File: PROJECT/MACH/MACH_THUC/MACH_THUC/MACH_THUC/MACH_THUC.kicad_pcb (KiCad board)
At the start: 2 copper layers, 177.8 x 99.1 mm, 66 parts, among them K1 SANYOU_SRD_Form_C, K2 SANYOU_SRD_Form_C, Q1 2SB688, Q2 BC547, Q3 BC547, U1 LM7805_TO220, U2 DS1307+, U3 LCD-016N002L, U4 PCF8574, U5 PC817, U6 PC817, Y1 Crystal 20M, Y2 Crystal 32.768KHz

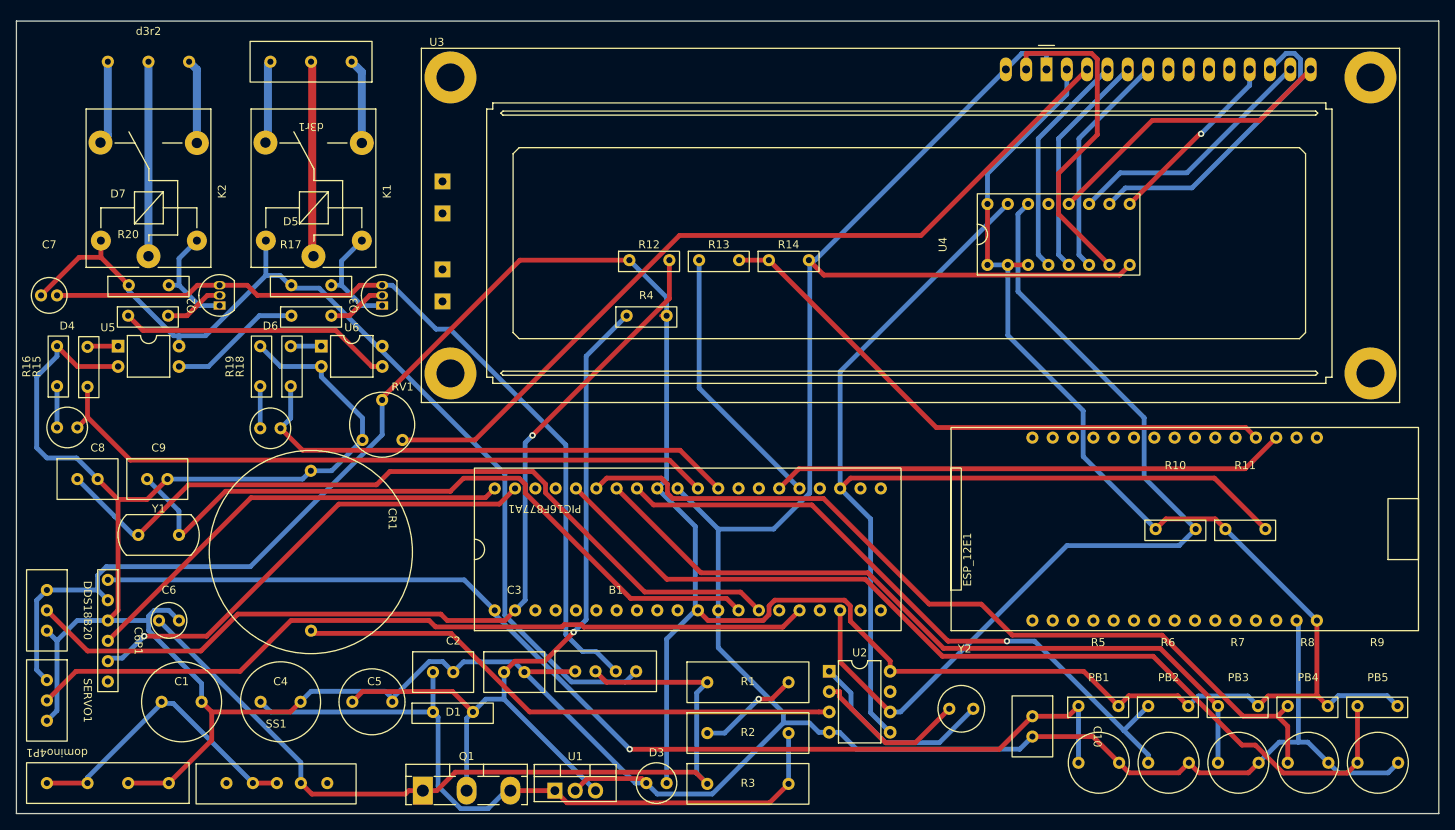
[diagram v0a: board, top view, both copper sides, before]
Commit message: update code'
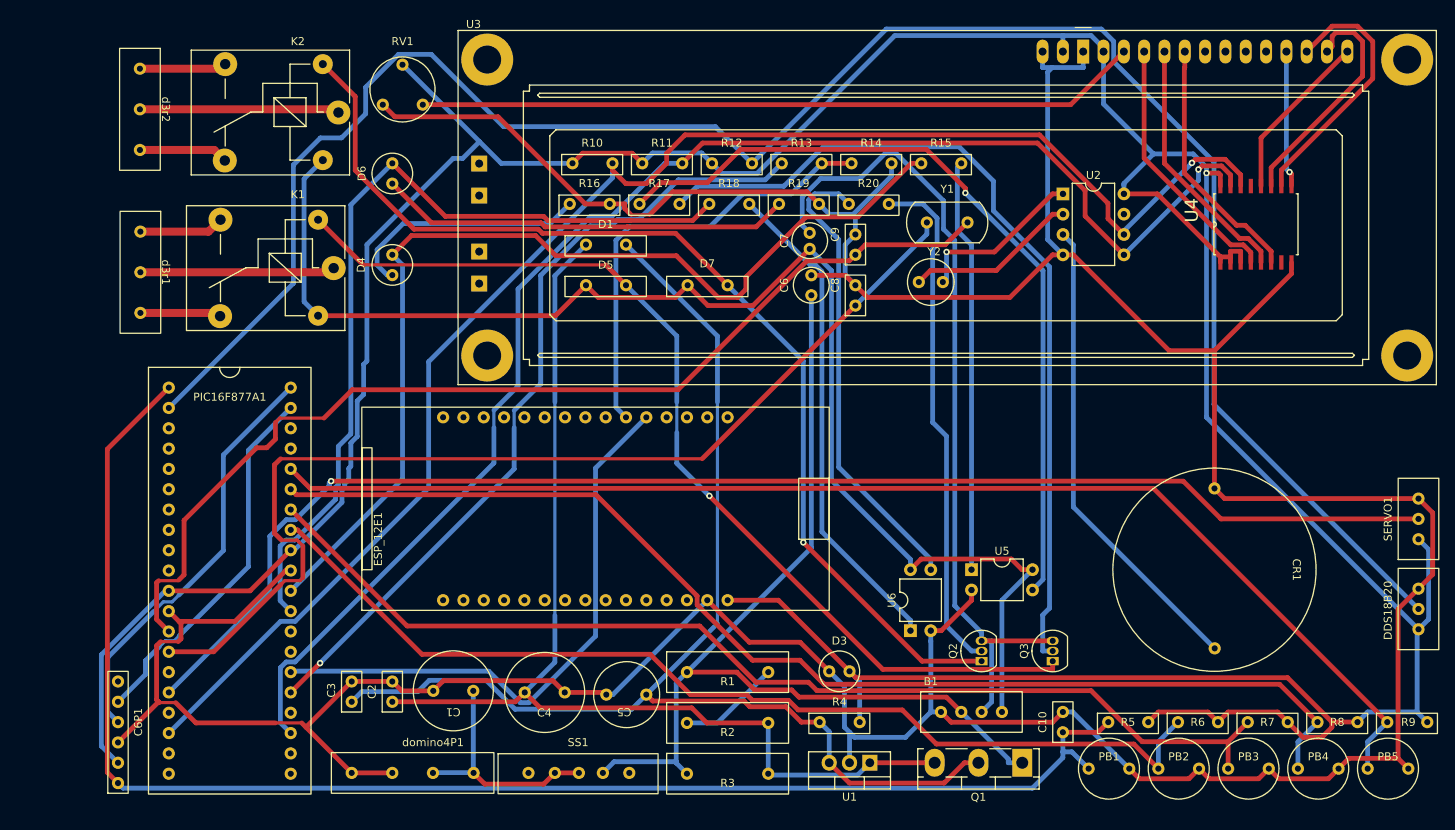
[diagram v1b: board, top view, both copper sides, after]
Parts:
- U4: footprint library_thuan_footprint:PCF8574 -> library_thuan_footprint:SOIC127P1032X265-16N
- d3r2: moved to F.Cu
- moved SERVO1 157.8 mm to (207.0, 113.0), turned to 90 degrees
- moved DDS18B20 156.2 mm to (207.0, 124.3), turned to 90 degrees
- moved R15 118.8 mm to (154.9, 61.1), turned to 0 degrees
- moved CR1 113.0 mm to (201.8, 119.4)
- moved U5 110.3 mm to (158.8, 119.4)
- moved Y1 106.0 mm to (155.7, 69.6)
- moved Q2 105.1 mm to (160.0, 130.8)
- moved Q3 94.9 mm to (168.9, 130.8)
- moved R20 91.2 mm to (145.9, 66.2)
- moved C7 89.2 mm to (132.7, 78.2), turned to 90 degrees
- moved C8 88.7 mm to (136.6, 83.8), turned to 90 degrees
- moved R10 86.1 mm to (111.3, 61.1)
- moved R11 86.1 mm to (120.1, 61.1)
- moved C6 82.2 mm to (132.5, 83.8), turned to 90 degrees
- moved U6 81.8 mm to (151.1, 127.0), turned to 90 degrees
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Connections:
- ESP_12E1 pad 18: rx -> unconnected-(ESP_12E1-TX-Pad18)
- ESP_12E1 pad 19: Net-(ESP_12E1-RX) -> unconnected-(ESP_12E1-RX-Pad19)
- ESP_12E1 pad 20: unconnected-(ESP_12E1-D8-Pad20) -> rx
- ESP_12E1 pad 21: unconnected-(ESP_12E1-D7-Pad21) -> Net-(ESP_12E1-D7)
- R13 pad 2: Net-(ESP_12E1-RX) -> Net-(ESP_12E1-D7)
- R14 pad 1: Net-(ESP_12E1-RX) -> Net-(ESP_12E1-D7)
- U3 pad 15: Net-(U3-A/VEE) -> +5V
- U4 pad 7: Net-(U3-A/VEE) -> unconnected-(U4-P3-Pad7)
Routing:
- net ds_18b20: track 115.2 -> 247.0 mm, vias 1 -> 0
- net Net-(D7-A): track 13.9 -> 132.0 mm, vias 0 -> 1
- net Net-(D5-A): track 14.0 -> 125.5 mm, vias 0 -> 1
- net Net-(Q3-B): track 7.40 -> 107.2 mm
- net +5V: track 391.0 -> 484.8 mm, vias 0 -> 1
- net Net-(R17-Pad1): track 16.7 -> 100.3 mm, vias 0 -> 1
- net scl: track 113.3 -> 191.3 mm, vias 0 -> 1
- net Net-(ESP_12E1-RX): track 73.8 -> 0.00 mm
- net servo: track 99.7 -> 173.4 mm, vias 0 -> 1
- net tx: track 33.7 -> 101.0 mm, vias 0 -> 1
- net Net-(R18-Pad2): track 3.82 -> 62.1 mm
- net Net-(Q2-B): track 7.48 -> 64.4 mm
- net Net-(ESP_12E1-D7): track 0.00 -> 56.1 mm
- net Net-(D1-A): track 104.8 -> 154.3 mm, vias 1 -> 0
- net Net-(R15-Pad2): track 3.86 -> 51.7 mm
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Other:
- board outline removed
